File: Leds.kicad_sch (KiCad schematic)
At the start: 16 parts, among them SW4 SW_SPDT, SW7 SW_Push

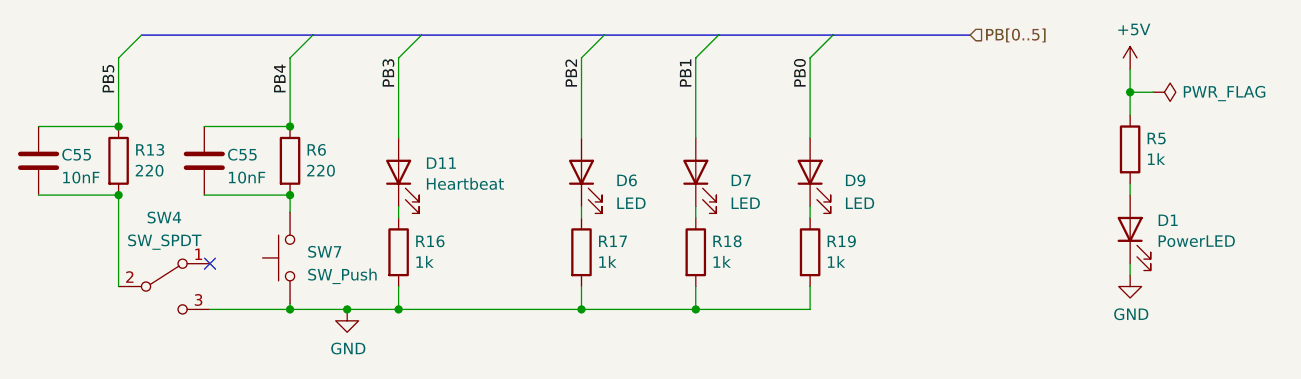
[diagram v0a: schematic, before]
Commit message: 40mm layout
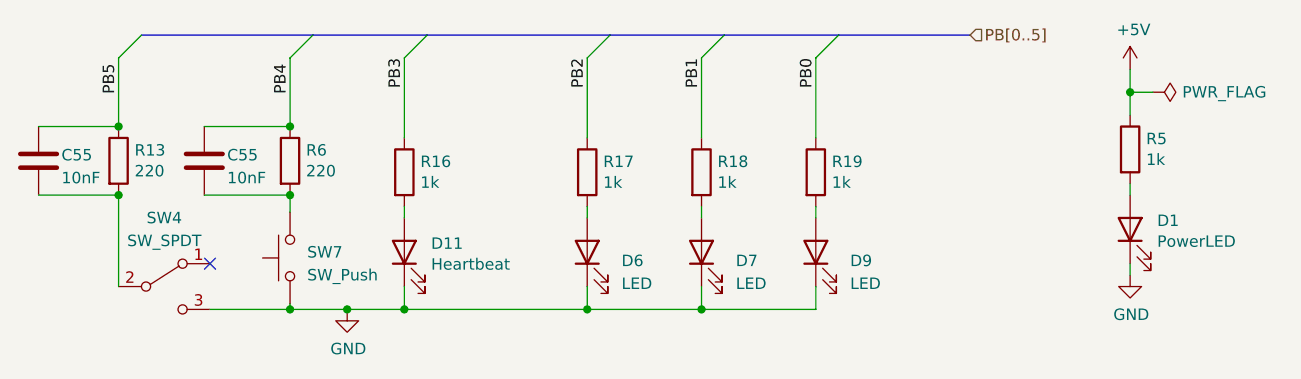
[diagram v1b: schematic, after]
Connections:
- net GND: now also D11.1 (K), D6.1 (K), D7.1 (K), D9.1 (K); no longer R16.2, R17.2, R18.2, R19.2
- net PB0: now also R19.1; no longer D9.2 (A)
- net PB1: now also R18.1; no longer D7.2 (A)
- net PB2: now also R17.1; no longer D6.2 (A)
- net PB3: now also R16.1; no longer D11.2 (A)
- new net: D7.2 (A), R18.2
- new net: D9.2 (A), R19.2
- new net: D11.2 (A), R16.2
- new net: D6.2 (A), R17.2
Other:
- moved on the sheet: D11, D6, D7, D9, R16, R17, R18, R19
